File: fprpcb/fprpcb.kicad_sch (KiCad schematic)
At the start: 46 parts, among them J1 Conn_02x04_Odd_Even, J2 Conn_01x02, J3 Conn_01x03, J4 Conn_01x03, J5 Conn_01x03, J6 Conn_01x03, J7 Conn_01x06, J8 Conn_01x04, SW1 Conn_01x02_Pin, SW2 Conn_01x02_Pin, SW3 Conn_01x02_Pin, SW4 Conn_01x02_Pin, SW5 Conn_01x02_Pin, SW6 Conn_01x02_Pin, U1 SC0918, U5 25LC1024-I/P

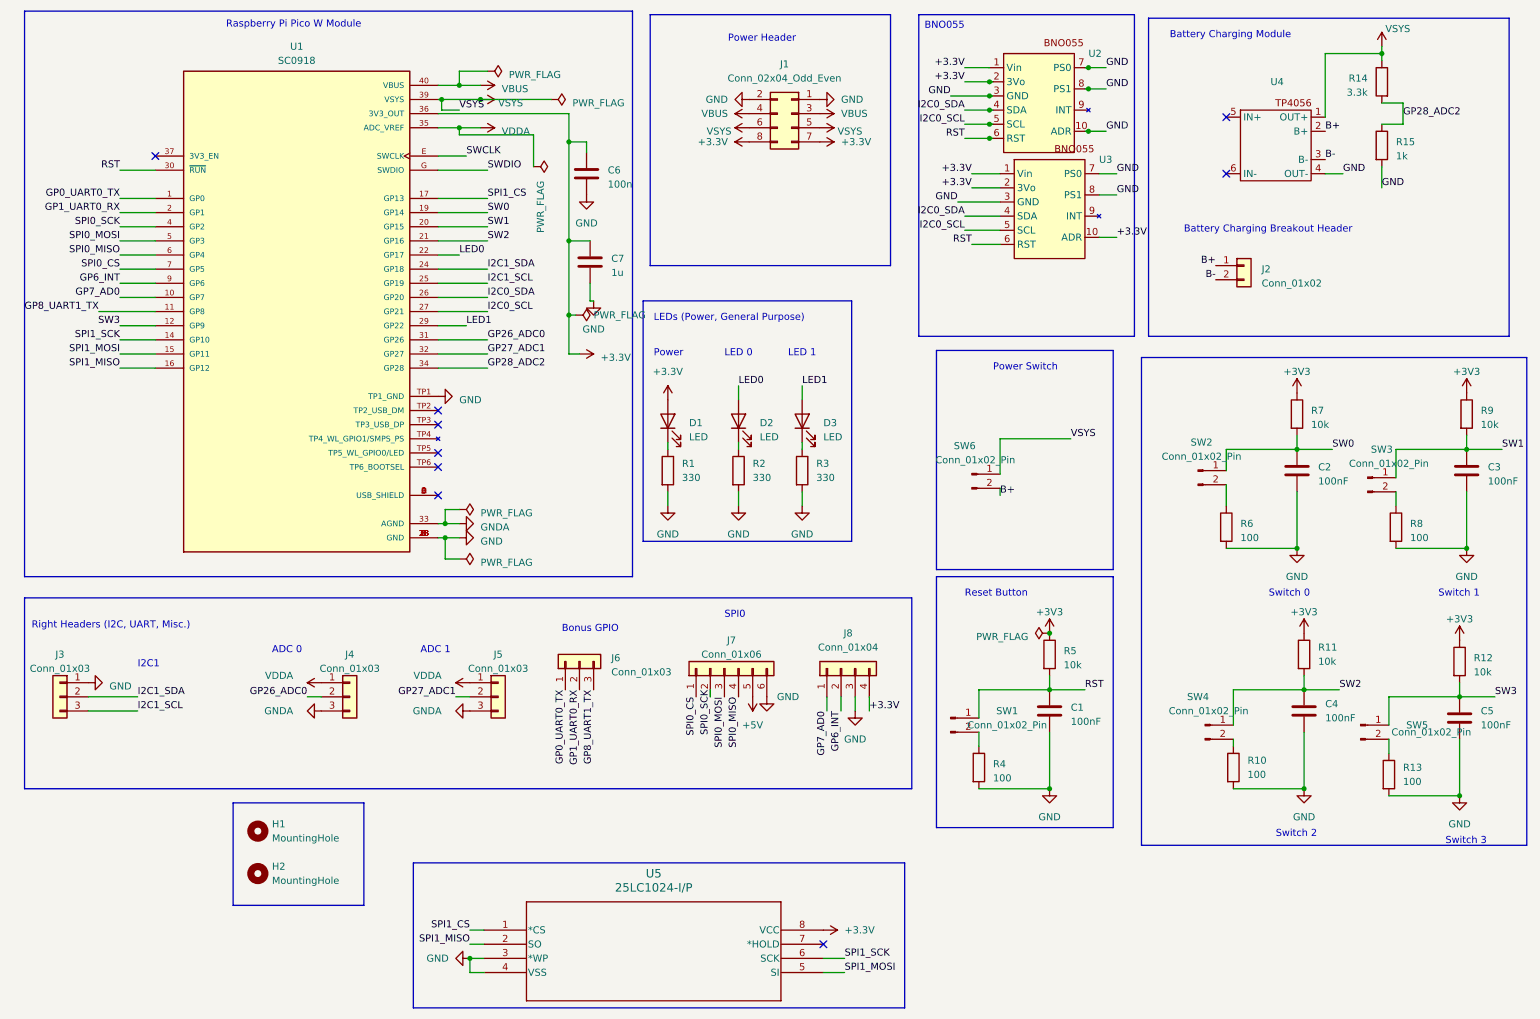
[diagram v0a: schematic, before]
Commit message: fprpcb
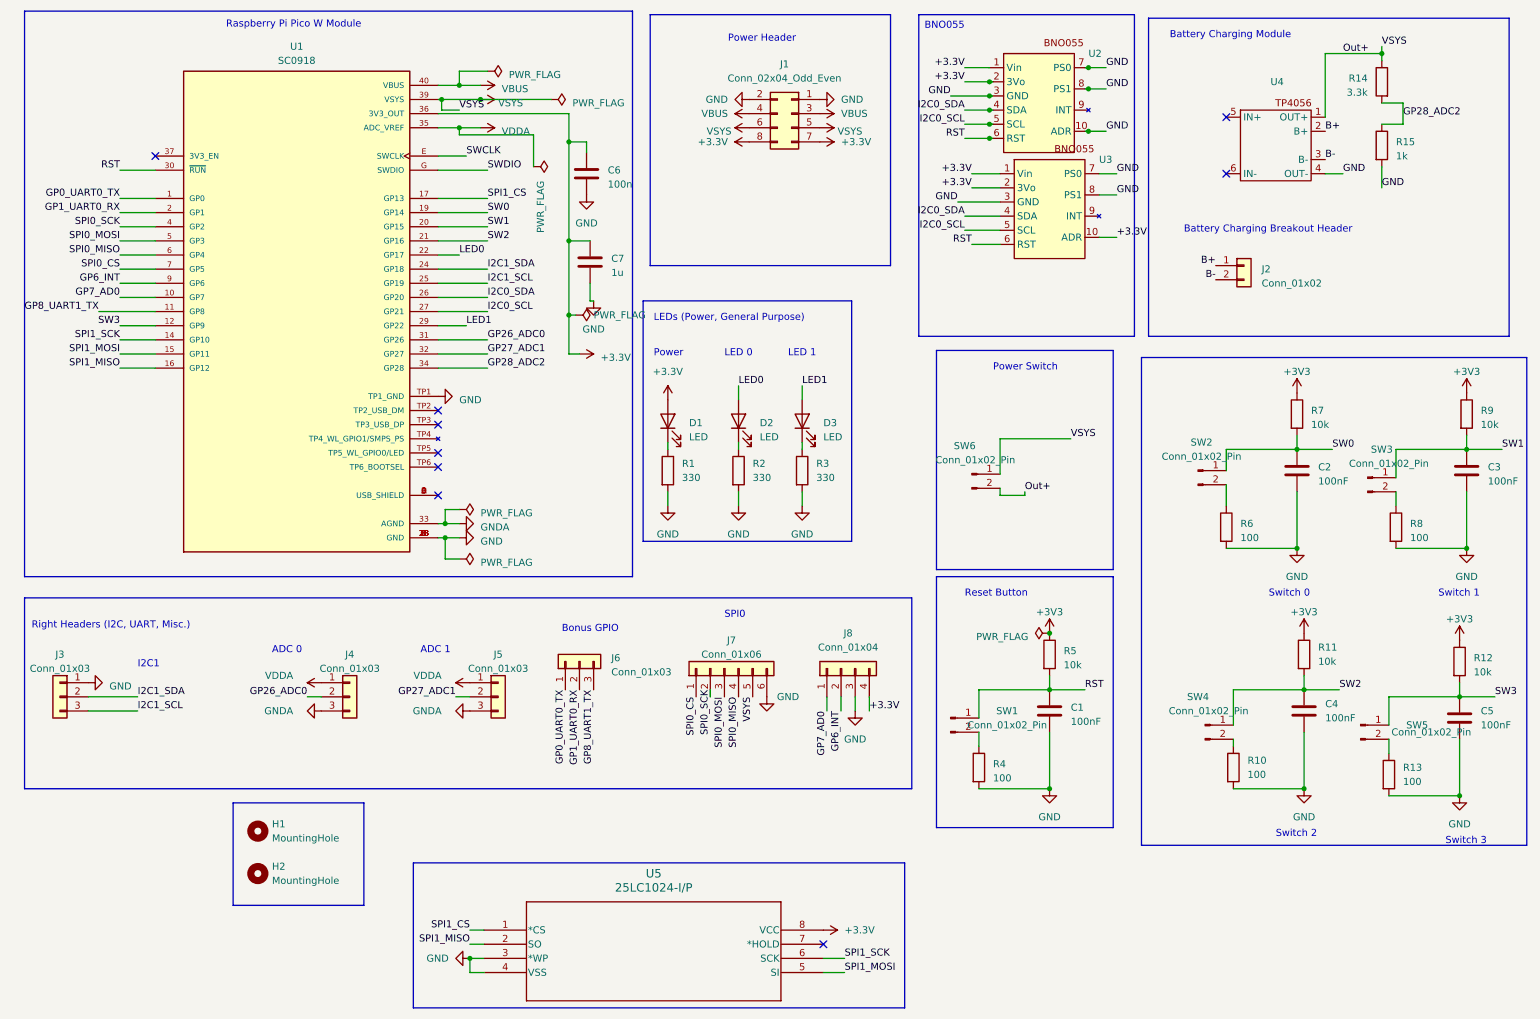
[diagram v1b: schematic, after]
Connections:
- net +5V: now also SW6.2 (Pin_2)
- net B+: no longer SW6.2 (Pin_2)
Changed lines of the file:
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@@
+    (stroke (width 0) (type default))
+  )
+  (wire (pts (xy 193.675 100.965) (xy 193.675 100.33))
     (stroke (width 0) (type default))
   )
@@
   )
   (wire (pts (xy 198.12 143.51) (xy 198.12 153.67))
+    (stroke (width 0) (type default))
+  )
+  (wire (pts (xy 189.23 100.965) (xy 193.675 100.965))
     (stroke (width 0) (type default))
   )
@@
     (effects (font (size 1.27 1.27)) (justify left bottom))
   )
-  (label "B+" (at 189.23 100.965 0) (fields_autoplaced)
-    (effects (font (size 1.27 1.27)) (justify left bottom))
-  )
   (label "GP1_UART0_RX" (at 31.115 50.165 180) (fields_autoplaced)
     (effects (font (size 1.27 1.27)) (justify right bottom))
@@
     (effects (font (size 1.27 1.27)) (justify left bottom))
   )
+  (label "VSYS" (at 257.81 20.32 0) (fields_autoplaced)
+    (effects (font (size 1.27 1.27)) (justify left bottom))
+  )
   (label "SWDIO" (at 97.155 42.545 0) (fields_autoplaced)
     (effects (font (size 1.27 1.27)) (justify left bottom))
@@
     (effects (font (size 1.27 1.27)) (justify left bottom))
   )
+  (label "VSYS" (at 144.78 137.16 270) (fields_autoplaced)
+    (effects (font (size 1.27 1.27)) (justify right bottom))
+  )
   (label "SPI0_SCK" (at 137.16 135.89 270) (fields_autoplaced)
     (effects (font (size 1.27 1.27)) (justify right bottom))
@@
     (effects (font (size 1.27 1.27)) (justify right bottom))
   )
+  (label "Out+" (at 193.675 100.33 0) (fields_autoplaced)
+    (effects (font (size 1.27 1.27)) (justify left bottom))
+  )
   (label "SW2" (at 97.155 55.245 0) (fields_autoplaced)
     (effects (font (size 1.27 1.27)) (justify left bottom))
@@
   )
   (label "GND" (at 208.28 35.56 0) (fields_autoplaced)
+    (effects (font (size 1.27 1.27)) (justify left bottom))
+  )
+  (label "Out+" (at 250.825 21.59 0) (fields_autoplaced)
     (effects (font (size 1.27 1.27)) (justify left bottom))
   )
@@
     )
   )
-  (symbol (lib_id "power:+5V") (at 144.78 137.16 180) (unit 1)
-    (in_bom yes) (on_board yes) (dnp no) (fields_autoplaced)
-    (property "Reference" "#PWR045" (at 144.78 133.35 0)
-      (effects (font (size 1.27 1.27)) hide)
-    )
-    (property "Value" "+5V" (at 144.78 142.24 0)
-      (effects (font (size 1.27 1.27)))
-    )
-    (property "Footprint" "" (at 144.78 137.16 0)
-      (effects (font (size 1.27 1.27)) hide)
-    )
-    (property "Datasheet" "" (at 144.78 137.16 0)
-      (effects (font (size 1.27 1.27)) hide)
-    )
-    (pin "1")
-    (instances
-      (project "fprpcb"
-        (path "/256b697e-9752-4e3a-a338-bc05701ab36e"
-          (reference "#PWR045") (unit 1)
-        )
-      )
-    )
-  )
   (symbol (lib_id "power:+3V3") (at 242.57 82.55 0) (unit 1)
     (in_bom yes) (on_board yes) (dnp no) (fields_autoplaced)
@@
         )
       )
-    )
-  )
-  (symbol (lib_id "power:+5V") (at 257.81 20.32 0) (unit 1)
-    (in_bom yes) (on_board yes) (dnp no)
-    (property "Reference" "#PWR032" (at 257.81 24.13 0)
-      (effects (font (size 1.27 1.27)) hide)
-    )
-    (property "Value" "VSYS" (at 258.445 17.145 0)
-      (effects (font (size 1.27 1.27)) (justify left))
-    )
-    (property "Footprint" "" (at 257.81 20.32 0)
-      (effects (font (size 1.27 1.27)) hide)
-    )
-    (property "Datasheet" "" (at 257.81 20.32 0)
-      (effects (font (size 1.27 1.27)) hide)
-    )
-    (pin "1")
-    (instances
-      (project "fprpcb"
-        (path "/256b697e-9752-4e3a-a338-bc05701ab36e"
-          (reference "#PWR032") (unit 1)
-        )
-      )

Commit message: Revert "fprpcb"
This reverts commit a24959e1a84143555ed98c59d3b6709d6d6878c6.
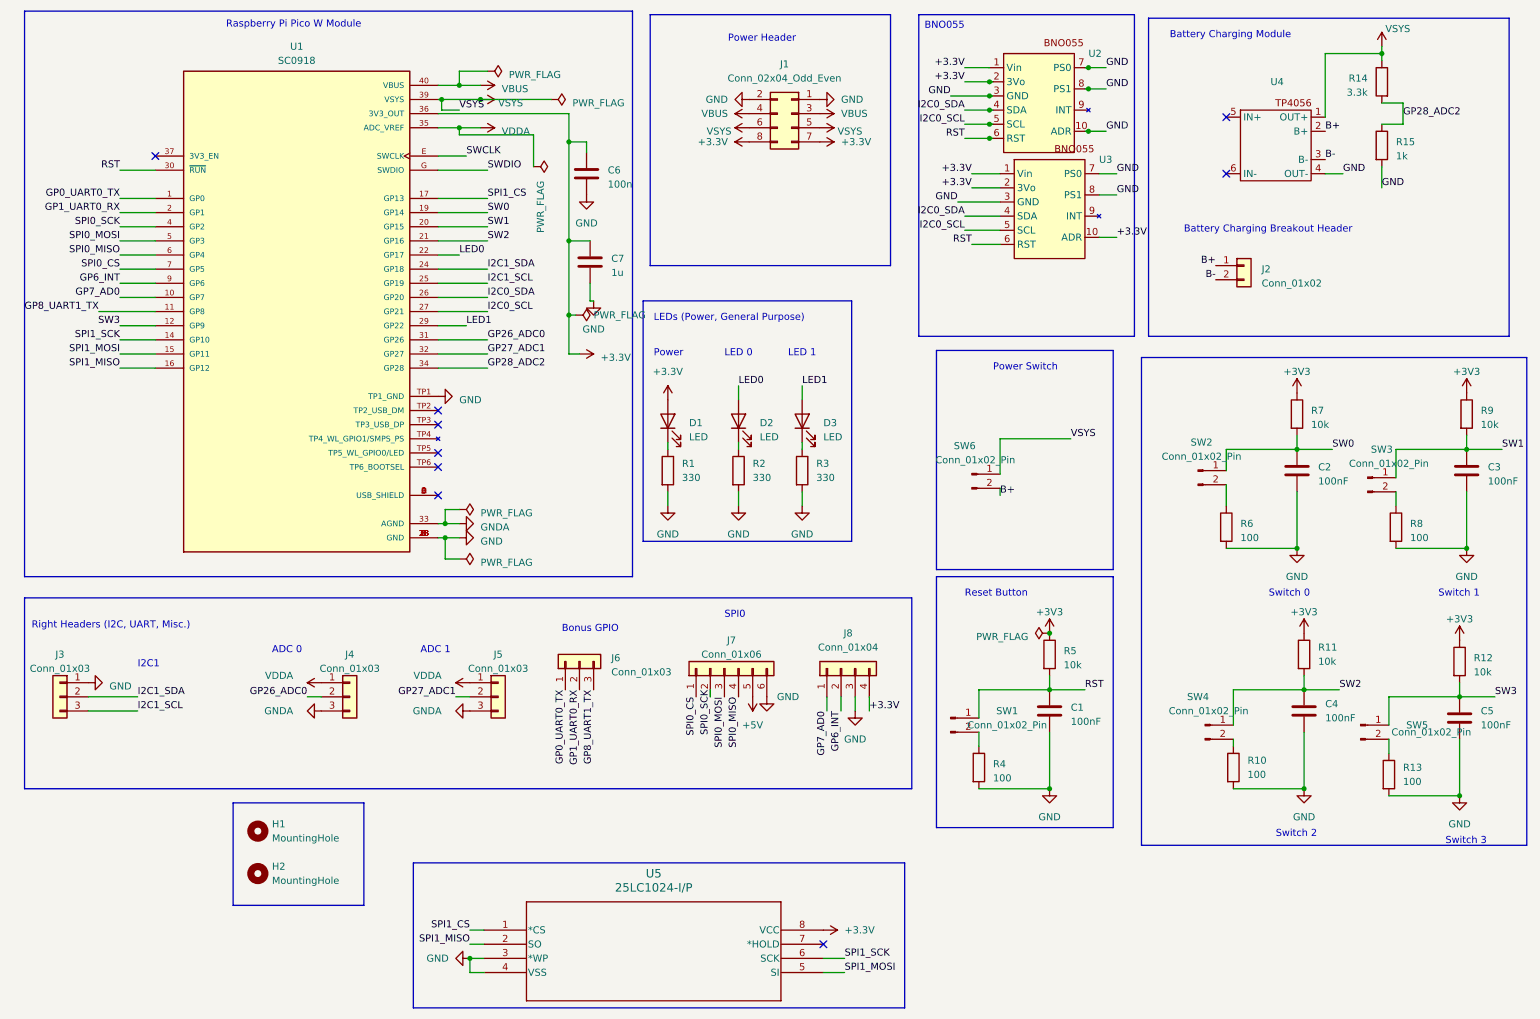
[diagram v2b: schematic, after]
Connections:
- net +5V: no longer SW6.2 (Pin_2)
- net B+: now also SW6.2 (Pin_2)
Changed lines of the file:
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@@
-    (stroke (width 0) (type default))
-  )
-  (wire (pts (xy 193.675 100.965) (xy 193.675 100.33))
     (stroke (width 0) (type default))
   )
@@
   )
   (wire (pts (xy 198.12 143.51) (xy 198.12 153.67))
-    (stroke (width 0) (type default))
-  )
-  (wire (pts (xy 189.23 100.965) (xy 193.675 100.965))
     (stroke (width 0) (type default))
   )
@@
     (effects (font (size 1.27 1.27)) (justify left bottom))
   )
+  (label "B+" (at 189.23 100.965 0) (fields_autoplaced)
+    (effects (font (size 1.27 1.27)) (justify left bottom))
+  )
   (label "GP1_UART0_RX" (at 31.115 50.165 180) (fields_autoplaced)
     (effects (font (size 1.27 1.27)) (justify right bottom))
@@
     (effects (font (size 1.27 1.27)) (justify left bottom))
   )
-  (label "VSYS" (at 257.81 20.32 0) (fields_autoplaced)
-    (effects (font (size 1.27 1.27)) (justify left bottom))
-  )
   (label "SWDIO" (at 97.155 42.545 0) (fields_autoplaced)
     (effects (font (size 1.27 1.27)) (justify left bottom))
@@
     (effects (font (size 1.27 1.27)) (justify left bottom))
   )
-  (label "VSYS" (at 144.78 137.16 270) (fields_autoplaced)
-    (effects (font (size 1.27 1.27)) (justify right bottom))
-  )
   (label "SPI0_SCK" (at 137.16 135.89 270) (fields_autoplaced)
     (effects (font (size 1.27 1.27)) (justify right bottom))
@@
     (effects (font (size 1.27 1.27)) (justify right bottom))
   )
-  (label "Out+" (at 193.675 100.33 0) (fields_autoplaced)
-    (effects (font (size 1.27 1.27)) (justify left bottom))
-  )
   (label "SW2" (at 97.155 55.245 0) (fields_autoplaced)
     (effects (font (size 1.27 1.27)) (justify left bottom))
@@
   )
   (label "GND" (at 208.28 35.56 0) (fields_autoplaced)
-    (effects (font (size 1.27 1.27)) (justify left bottom))
-  )
-  (label "Out+" (at 250.825 21.59 0) (fields_autoplaced)
     (effects (font (size 1.27 1.27)) (justify left bottom))
   )
@@
     )
   )
+  (symbol (lib_id "power:+5V") (at 144.78 137.16 180) (unit 1)
+    (in_bom yes) (on_board yes) (dnp no) (fields_autoplaced)
+    (property "Reference" "#PWR045" (at 144.78 133.35 0)
+      (effects (font (size 1.27 1.27)) hide)
+    )
+    (property "Value" "+5V" (at 144.78 142.24 0)
+      (effects (font (size 1.27 1.27)))
+    )
+    (property "Footprint" "" (at 144.78 137.16 0)
+      (effects (font (size 1.27 1.27)) hide)
+    )
+    (property "Datasheet" "" (at 144.78 137.16 0)
+      (effects (font (size 1.27 1.27)) hide)
+    )
+    (pin "1")
+    (instances
+      (project "fprpcb"
+        (path "/256b697e-9752-4e3a-a338-bc05701ab36e"
+          (reference "#PWR045") (unit 1)
+        )
+      )
+    )
+  )
   (symbol (lib_id "power:+3V3") (at 242.57 82.55 0) (unit 1)
     (in_bom yes) (on_board yes) (dnp no) (fields_autoplaced)
@@
         )
       )
+    )
+  )
+  (symbol (lib_id "power:+5V") (at 257.81 20.32 0) (unit 1)
+    (in_bom yes) (on_board yes) (dnp no)
+    (property "Reference" "#PWR032" (at 257.81 24.13 0)
+      (effects (font (size 1.27 1.27)) hide)
+    )
+    (property "Value" "VSYS" (at 258.445 17.145 0)
+      (effects (font (size 1.27 1.27)) (justify left))
+    )
+    (property "Footprint" "" (at 257.81 20.32 0)
+      (effects (font (size 1.27 1.27)) hide)
+    )
+    (property "Datasheet" "" (at 257.81 20.32 0)
+      (effects (font (size 1.27 1.27)) hide)
+    )
+    (pin "1")
+    (instances
+      (project "fprpcb"
+        (path "/256b697e-9752-4e3a-a338-bc05701ab36e"
+          (reference "#PWR032") (unit 1)
+        )
+      )
